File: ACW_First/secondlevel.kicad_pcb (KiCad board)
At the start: 2 copper layers, 103 x 65 mm, 69 parts, among them J11 24VDC, J12 Conn_01x02_Pin, J13 Conn_01x04_Socket, J14 Conn_01x02_Pin, J2 Conn_01x03_Pin, J3 3.8VDC, J4 5VDC, J5 12VDC, U2 MP1584EN, U3 MP1584EN

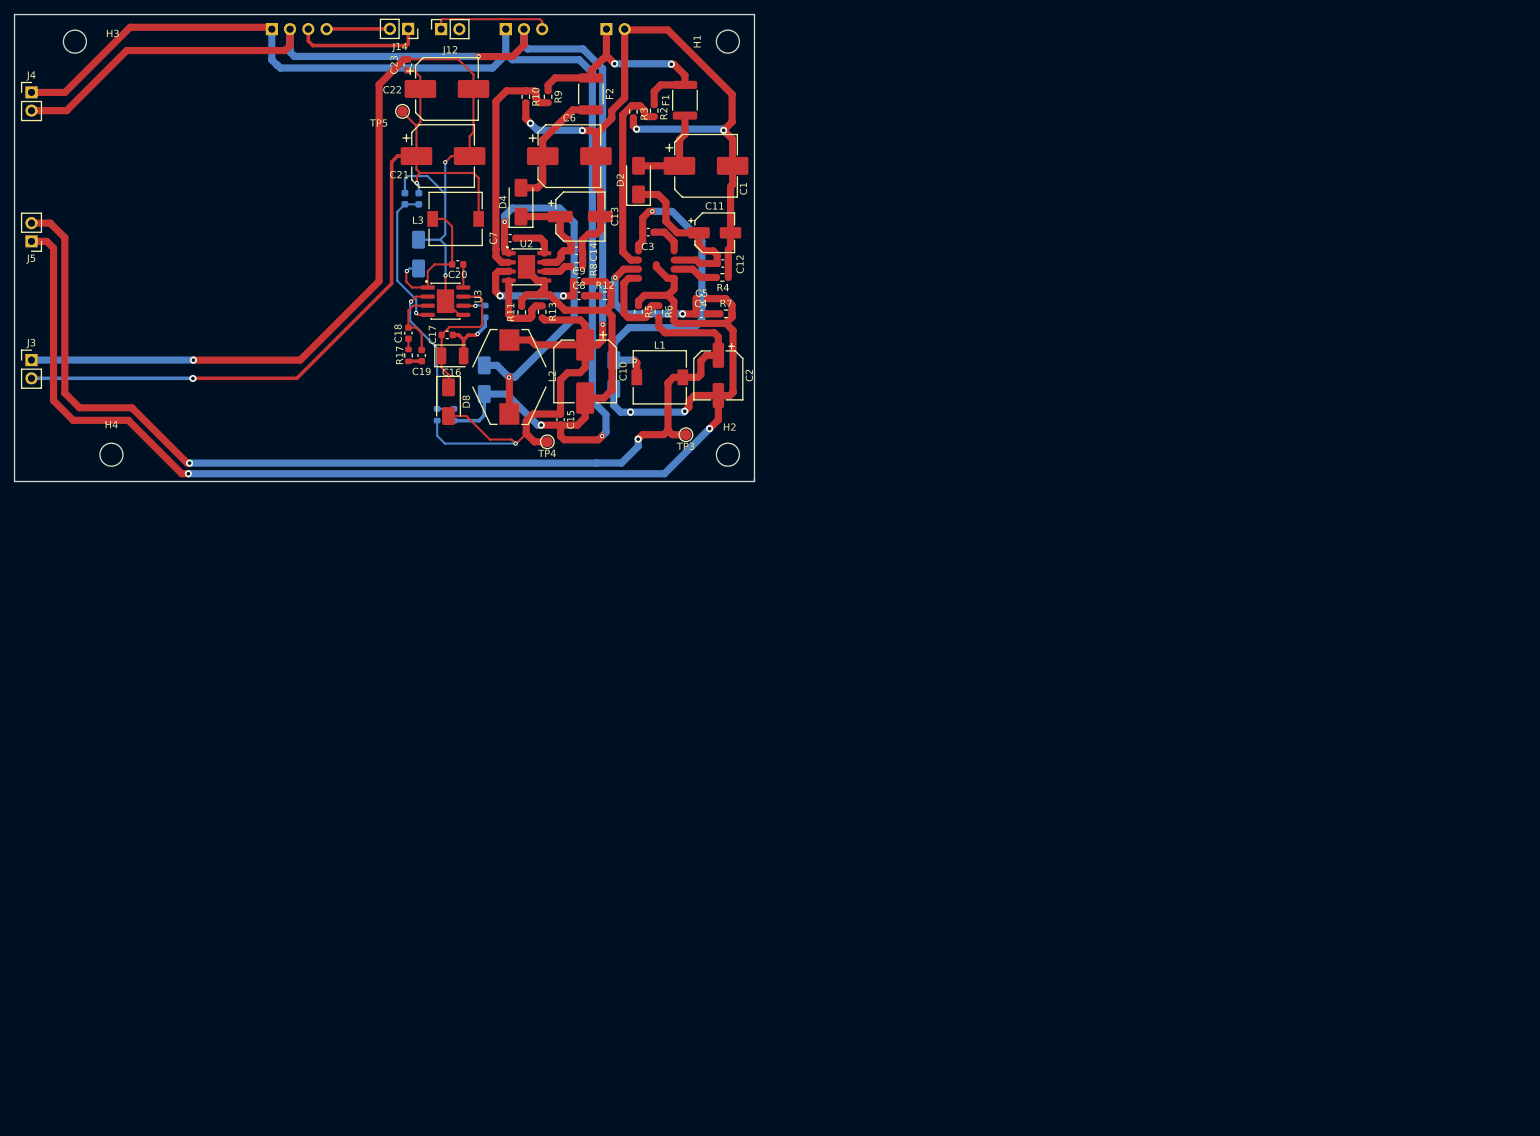
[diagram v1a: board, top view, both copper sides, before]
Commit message: okok
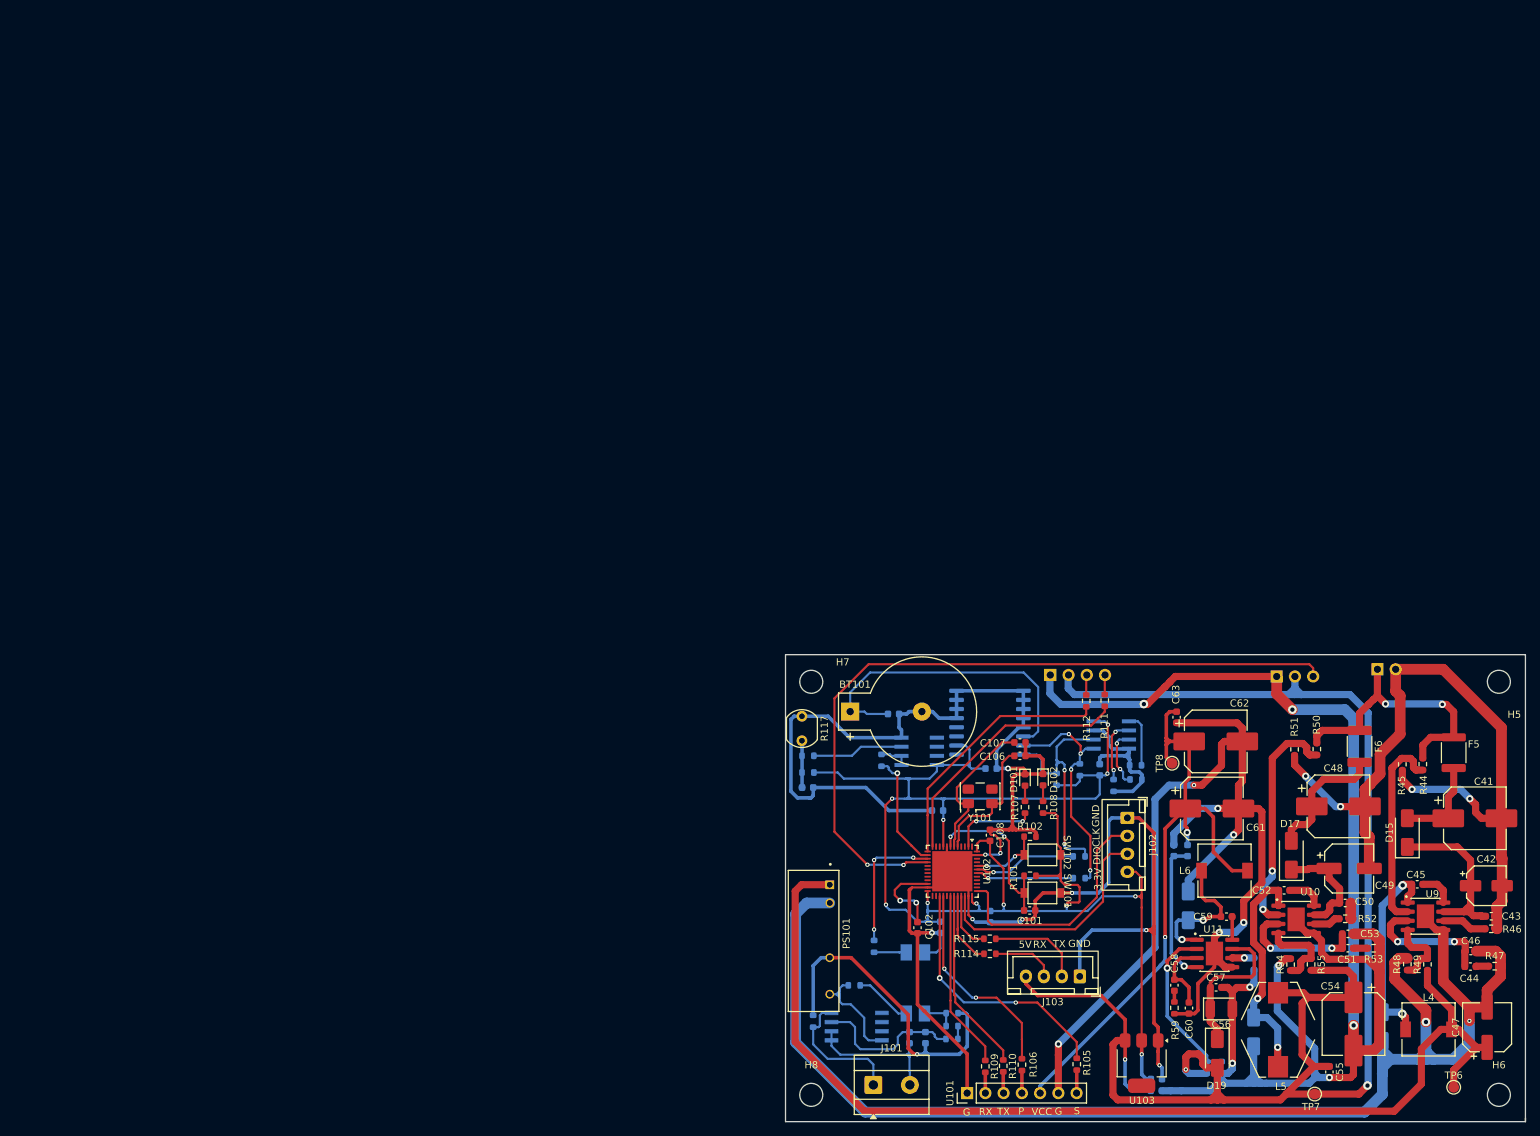
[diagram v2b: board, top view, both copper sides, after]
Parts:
- removed C1, C6: 220µF, Capacitor_SMD:CP_Elec_8x10.5
- removed C10: 470µF, Capacitor_SMD:CP_Elec_8x10.5
- removed C11: 10µF, Capacitor_SMD:CP_Elec_5x5.4
- removed C12, C14, C15, C17, C20, C23, C3, C7: 100nF, Capacitor_SMD:C_0603_1608Metric
- removed C13: 10µF, Capacitor_SMD:CP_Elec_6.3x5.4
- removed C16: 10µF, Capacitor_Tantalum_SMD:CP_EIA-3528-21_Kemet-B
- removed C18, C4, C8: 220pF, Capacitor_SMD:C_0603_1608Metric
- removed C19, C5, C9: NS, Capacitor_SMD:C_0603_1608Metric
- removed C2: 22µF, Capacitor_SMD:CP_Elec_6.3x5.4
- removed C21, C22: 330µF, Capacitor_SMD:CP_Elec_8x10.5
- removed D2, D3, D4, D5, D7, D8: SS34, Diode_SMD:D_SMA
- removed F1: Resettable Fuse/2A, Fuse:Fuse_1812_4532Metric
- removed F2: Resettable Fuse/2A, Fuse:Fuse_1812_4532Metric_Pad1.30x3.40mm_HandSolder
- removed H1, H2, H3, H4: MountingHole, MountingHole:MountingHole_3.2mm_M3
- removed J12, J14: Conn_01x02_Pin, Connector_PinSocket_2.54mm:PinSocket_1x02_P2.54mm_Vertical
- removed J3: 3.8VDC, Connector_PinHeader_2.54mm:PinHeader_1x02_P2.54mm_Vertical
- removed J4: 5VDC, Connector_PinHeader_2.54mm:PinHeader_1x02_P2.54mm_Vertical
- removed J5: 12VDC, Connector_PinHeader_2.54mm:PinHeader_1x02_P2.54mm_Vertical
- removed L1: 22µH, Inductor_SMD:L_7.3x7.3_H4.5
- removed L2: 10µH, Inductor_SMD:L_Bourns-SRR1005
- removed L3: 10µH, Inductor_SMD:L_7.3x7.3_H4.5
- removed R10: 11KΩ, Resistor_SMD:R_0603_1608Metric
- removed R11, R5: 40.2KΩ, Resistor_SMD:R_0603_1608Metric
- removed R12, R17: 68.1KΩ, Resistor_SMD:R_0603_1608Metric
- removed R13: 210KΩ, Resistor_SMD:R_0603_1608Metric
- removed R14: 20KΩ, Resistor_SMD:R_0603_1608Metric
- removed R15: 10KΩ, Resistor_SMD:R_0603_1608Metric
- removed R16, R4, R8: 200KΩ, Resistor_SMD:R_0603_1608Metric
- removed R18: 150KΩ, Capacitor_SMD:C_0603_1608Metric
- removed R19: 40.2KΩ, Capacitor_SMD:C_0603_1608Metric
- removed R2: 149KΩ/1%, Resistor_SMD:R_0603_1608Metric
- removed R3: 11KΩ/1%, Resistor_SMD:R_0603_1608Metric
- removed R6: 562KΩ, Resistor_SMD:R_0603_1608Metric
- removed R7: 68.1KΩ/1%, Resistor_SMD:R_0603_1608Metric
- removed R9: 149KΩ, Resistor_SMD:R_0603_1608Metric
- removed TP3: 12VTP, TestPoint:TestPoint_Pad_D1.5mm
- removed TP4: 5VTP, TestPoint:TestPoint_Pad_D1.5mm
- removed TP5: 3.8VTP, TestPoint:TestPoint_Pad_D1.5mm
- removed U2, U3: MP1584EN, Custom_Footprints:SOIC127P600X170-9N
- added BT101: Battery_Cell, Battery:BatteryHolder_Keystone_500, F.Cu at (550.6, 238.5)
- added C101: 100nf, Capacitor_SMD:C_0603_1608Metric, F.Cu at (575.6, 266.2)
- added C102: 2.2uf, Capacitor_SMD:C_0603_1608Metric, F.Cu at (559.9, 268.6)
- added C103: 100nf, Capacitor_SMD:C_0603_1608Metric, B.Cu at (593.2, 291.3)
- added C104: 100nf, Capacitor_SMD:C_0603_1608Metric, B.Cu at (563.1, 268.6)
- added C105: 100nf, Capacitor_SMD:C_0603_1608Metric, B.Cu at (570.0, 267.1)
- added C106: 22pf, Capacitor_SMD:C_0603_1608Metric, F.Cu at (574.2, 244.7)
- added C107: 22pf, Capacitor_SMD:C_0603_1608Metric, F.Cu at (574.2, 242.8)
- added C108: 100nf, Capacitor_SMD:C_0603_1608Metric, F.Cu at (570.0, 255.7)
- added C109: 100nf, Capacitor_SMD:C_0603_1608Metric, B.Cu at (593.2, 289.7)
- added C110: 100nf, Capacitor_SMD:C_0603_1608Metric, B.Cu at (562.7, 252.3)
- added C111: 100nf, Capacitor_SMD:C_0603_1608Metric, B.Cu at (544.6, 249.1)
- added C112: 1uf, Capacitor_SMD:C_0603_1608Metric, B.Cu at (570.2, 246.5)
- added C113: 1uf, Capacitor_SMD:C_0603_1608Metric, B.Cu at (585.3, 246.6)
- added C114: 1uf, Capacitor_SMD:C_0603_1608Metric, B.Cu at (556.6, 238.9)
- added C115: 1uf, Capacitor_SMD:C_0603_1608Metric, B.Cu at (561.0, 283.9)
- added C116: 1uf, Capacitor_SMD:C_0603_1608Metric, B.Cu at (558.8, 283.9)
- added C41: 220µF, Capacitor_SMD:CP_Elec_8x10.5, F.Cu at (637.5, 253.4)
- added C42: 10µF, Capacitor_SMD:CP_Elec_5x5.4, F.Cu at (639.1, 262.8)
- added C43: 100nF, Capacitor_SMD:C_0603_1608Metric, F.Cu at (639.8, 267.0)
- added C44: 220pF, Capacitor_SMD:C_0603_1608Metric, F.Cu at (636.9, 274.0)
- added C45: 100nF, Capacitor_SMD:C_0603_1608Metric, F.Cu at (629.5, 262.6)
- added C46: NS, Capacitor_SMD:C_0603_1608Metric, F.Cu at (637.0, 271.9)
- added C47: 22µF, Capacitor_SMD:CP_Elec_6.3x5.4, F.Cu at (639.2, 282.5)
- added C48: 220µF, Capacitor_SMD:CP_Elec_8x10.5, F.Cu at (618.5, 251.7)
- added C49: 10µF, Capacitor_SMD:CP_Elec_6.3x5.4, F.Cu at (620.0, 260.4)
- added C50: 100nF, Capacitor_SMD:C_0603_1608Metric, F.Cu at (619.5, 265.2)
- added C51: 220pF, Capacitor_SMD:C_0603_1608Metric, F.Cu at (619.9, 271.5)
- added C52: 100nF, Capacitor_SMD:C_0603_1608Metric, F.Cu at (611.0, 263.4)
- added C53: NS, Capacitor_SMD:C_0603_1608Metric, F.Cu at (619.9, 269.5)
- added C54: 470µF, Capacitor_SMD:CP_Elec_8x10.5, F.Cu at (620.6, 282.0)
- added C55: 100nF, Capacitor_SMD:C_0603_1608Metric, F.Cu at (617.3, 288.7)
- added C56: 10µF, Capacitor_Tantalum_SMD:CP_EIA-3528-21_Kemet-B, F.Cu at (602.2, 279.9)
- added C57: 100nF, Capacitor_SMD:C_0603_1608Metric, F.Cu at (601.5, 276.9)
- added C58: 220pF, Capacitor_SMD:C_0603_1608Metric, F.Cu at (595.7, 276.6)
- added C59: 100nF, Capacitor_SMD:C_0603_1608Metric, F.Cu at (603.0, 267.1)
- added C60: NS, Capacitor_SMD:C_0603_1608Metric, F.Cu at (597.7, 279.8)
- added C61: 330µF, Capacitor_SMD:CP_Elec_8x10.5, F.Cu at (600.9, 252.0)
- added C62: 330µF, Capacitor_SMD:CP_Elec_8x10.5, F.Cu at (601.5, 242.7)
- added C63: 100nF, Capacitor_SMD:C_0603_1608Metric, F.Cu at (596.0, 239.3)
- added D101: LED, LED_SMD:LED_0603_1608Metric, F.Cu at (574.9, 248.0)
- added D102: LED, LED_SMD:LED_0603_1608Metric, F.Cu at (577.4, 248.0)
- added D15: SS34, Diode_SMD:D_SMA, F.Cu at (628.1, 255.4)
- added D16: SS34, Diode_SMD:D_SMA, B.Cu at (624.6, 282.4)
- added D17: SS34, Diode_SMD:D_SMA, F.Cu at (612.0, 258.5)
- added D18: SS34, Diode_SMD:D_SMA, B.Cu at (606.7, 283.1)
- added D19: SS34, Diode_SMD:D_SMA, F.Cu at (601.7, 286.1)
- added D20: SS34, Diode_SMD:D_SMA, B.Cu at (597.6, 265.6)
- added F5: Resettable Fuse/2A, Fuse:Fuse_1812_4532Metric, F.Cu at (634.6, 244.2)
- added F6: Resettable Fuse/2A, Fuse:Fuse_1812_4532Metric_Pad1.30x3.40mm_HandSolder, F.Cu at (621.5, 243.4)
- added H5: MountingHole, MountingHole:MountingHole_3.2mm_M3, F.Cu at (640.9, 234.4)
- added H6: MountingHole, MountingHole:MountingHole_3.2mm_M3, F.Cu at (640.9, 291.9)
- added H7: MountingHole, MountingHole:MountingHole_3.2mm_M3, F.Cu at (545.2, 234.4)
- added H8: MountingHole, MountingHole:MountingHole_3.2mm_M3, F.Cu at (545.2, 291.9)
- added J101: Conn_01x02_Male, TerminalBlock_MetzConnect:TerminalBlock_MetzConnect_Type101_RT01602HBWC_1x02_P5.08mm_Horizontal, F.Cu at (553.8, 290.5)
- added J102: Conn_STLink, Connector_JST:JST_XH_B4B-XH-A_1x04_P2.50mm_Vertical, F.Cu at (589.1, 253.3)
- added J103: Conn_01x04_Female, Connector_JST:JST_XH_B4B-XH-A_1x04_P2.50mm_Vertical, F.Cu at (582.5, 275.4)
- added L4: 22µH, Inductor_SMD:L_7.3x7.3_H4.5, F.Cu at (631.1, 282.8)
- added L5: 10µH, Inductor_SMD:L_Bourns-SRR1005, F.Cu at (610.1, 282.8)
- added L6: 10µH, Inductor_SMD:L_7.3x7.3_H4.5, F.Cu at (602.7, 260.7)
- added PS101: RKZ-1212S_P, Custom_Library:CONV_RKZ-1212S_P, F.Cu at (545.5, 270.5)
- added R101: 10k, Resistor_SMD:R_0603_1608Metric, F.Cu at (575.6, 261.4)
- added R102: 10k, Resistor_SMD:R_0603_1608Metric, F.Cu at (575.6, 255.9)
- added R103: 100, Resistor_SMD:R_0603_1608Metric, B.Cu at (582.5, 261.7)
- added R104: 100, Resistor_SMD:R_0603_1608Metric, B.Cu at (582.4, 258.7)
- added R105: 100, Resistor_SMD:R_0603_1608Metric, F.Cu at (582.1, 287.6)
- added R106: 100, Resistor_SMD:R_0603_1608Metric, F.Cu at (574.5, 287.7)
- added R107: 220, Resistor_SMD:R_0603_1608Metric, F.Cu at (574.9, 251.8)
- added R108: 220, Resistor_SMD:R_0603_1608Metric, F.Cu at (577.4, 251.8)
- added R109: 100, Resistor_SMD:R_0603_1608Metric, F.Cu at (569.4, 287.9)
- added R110: 100, Resistor_SMD:R_0603_1608Metric, F.Cu at (571.9, 287.8)
- added R111: 100, Resistor_SMD:R_0603_1608Metric, F.Cu at (586.0, 237.0)
- added R112: 100, Resistor_SMD:R_0603_1608Metric, F.Cu at (583.4, 237.0)
- added R113: 100, Resistor_SMD:R_0603_1608Metric, B.Cu at (554.9, 245.3)
- added R114: 100, Resistor_SMD:R_0603_1608Metric, F.Cu at (570.0, 272.2)
- added R115: 100, Resistor_SMD:R_0603_1608Metric, F.Cu at (570.0, 270.2)
- added R116: 10k, Resistor_SMD:R_0603_1608Metric, B.Cu at (544.7, 247.0)
- added R117: LDR07, OptoDevice:R_LDR_5.1x4.3mm_P3.4mm_Vertical, F.Cu at (543.9, 242.6)
- added R118: 220, Resistor_SMD:R_0603_1608Metric, B.Cu at (544.7, 244.7)
- added R119: 4.7k, Resistor_SMD:R_0603_1608Metric, B.Cu at (590.4, 248.0)
- added R120: 4.7k, Resistor_SMD:R_0603_1608Metric, B.Cu at (587.2, 248.8)
- added R121: 4.7k, Resistor_SMD:R_0603_1608Metric, B.Cu at (590.3, 246.0)
- added R122: 4.7k, Resistor_SMD:R_0603_1608Metric, B.Cu at (582.5, 246.6)
- added R123: 4.7k, Resistor_SMD:R_0603_1608Metric, B.Cu at (579.3, 248.0)
- added R124: 220, Resistor_SMD:R_0603_1608Metric, B.Cu at (553.9, 271.2)
- added R125: 10k, Resistor_SMD:R_0603_1608Metric, B.Cu at (551.1, 276.6)
- added R126: 4.7k, Resistor_SMD:R_0603_1608Metric, B.Cu at (564.8, 280.5)
- added R127: 10k, Resistor_SMD:R_0603_1608Metric, B.Cu at (564.8, 282.3)
- added R128: 10k, Resistor_SMD:R_0603_1608Metric, B.Cu at (564.7, 284.1)
- added R129: 4.7k, Resistor_SMD:R_0603_1608Metric, B.Cu at (545.4, 281.6)
- added R44: 149KΩ/1%, Resistor_SMD:R_0603_1608Metric, F.Cu at (630.3, 245.8)
- added R45: 11KΩ/1%, Resistor_SMD:R_0603_1608Metric, F.Cu at (627.4, 245.9)
- added R46: 200KΩ, Resistor_SMD:R_0603_1608Metric, F.Cu at (639.8, 268.8)
- added R47: 68.1KΩ/1%, Resistor_SMD:R_0603_1608Metric, F.Cu at (640.3, 274.0)
- added R48: 40.2KΩ, Resistor_SMD:R_0603_1608Metric, F.Cu at (628.1, 273.7)
- added R49: 562KΩ, Resistor_SMD:R_0603_1608Metric, F.Cu at (630.9, 273.7)
- added R50: 149KΩ, Resistor_SMD:R_0603_1608Metric, F.Cu at (615.5, 243.7)
- added R51: 11KΩ, Resistor_SMD:R_0603_1608Metric, F.Cu at (612.4, 243.8)
- added R52: 200KΩ, Resistor_SMD:R_0603_1608Metric, F.Cu at (619.5, 267.4)
- added R53: 68.1KΩ, Resistor_SMD:R_0603_1608Metric, F.Cu at (623.4, 271.5)
- added R54: 40.2KΩ, Resistor_SMD:R_0603_1608Metric, F.Cu at (611.9, 273.7)
- added R55: 210KΩ, Resistor_SMD:R_0603_1608Metric, F.Cu at (614.7, 273.7)
- added R56: 20KΩ, Resistor_SMD:R_0603_1608Metric, B.Cu at (600.2, 288.1)
- added R57: 10KΩ, Resistor_SMD:R_0603_1608Metric, B.Cu at (602.3, 288.1)
- added R58: 200KΩ, Resistor_SMD:R_0603_1608Metric, B.Cu at (606.8, 273.6)
- added R59: 68.1KΩ, Resistor_SMD:R_0603_1608Metric, F.Cu at (595.7, 279.8)
- added R60: 40.2KΩ, Capacitor_SMD:C_0603_1608Metric, B.Cu at (595.6, 257.9)
- added R61: 150KΩ, Capacitor_SMD:C_0603_1608Metric, B.Cu at (597.5, 257.9)
- added SW101: SW_Push, Library:Pushbutton_3x4x2mm_2P_SMD, F.Cu at (577.3, 261.3)
- added SW102: SW_Push, Library:Pushbutton_3x4x2mm_2P_SMD, F.Cu at (577.3, 256.0)
- added TP6: 12VTP, TestPoint:TestPoint_Pad_D1.5mm, F.Cu at (634.6, 290.8)
- added TP7: 5VTP, TestPoint:TestPoint_Pad_D1.5mm, F.Cu at (615.2, 291.8)
- added TP8: 3.8VTP, TestPoint:TestPoint_Pad_D1.5mm, F.Cu at (595.4, 245.7)
- added U10: MP1584EN, Custom_Footprints:SOIC127P600X170-9N, F.Cu at (612.7, 267.5)
- added U101: A7600_Pinout, Connector_PinHeader_2.54mm:PinHeader_1x07_P2.54mm_Vertical, F.Cu at (566.9, 291.6)
- added U102: STM32F401CCUx, Package_DFN_QFN:QFN-48-1EP_7x7mm_P0.5mm_EP5.6x5.6mm, F.Cu at (564.8, 260.8)
- added U103: AMS1117-3.3, Package_TO_SOT_SMD:SOT-223, F.Cu at (591.1, 287.5)
- added U104: MCP6002-I_SN, Custom_Library:SOIC127P600X175-8N, B.Cu at (560.2, 244.1)
- added U105: DS3231M, Package_SO:SOIC-16W_7.5x10.3mm_P1.27mm, B.Cu at (570.0, 240.1)
- added U106: AT24C512-SSHM, Custom_Library:SOIC127P600X175-8N, B.Cu at (586.9, 241.8)
- added U107: PC817, Custom_Library:SOP254P975X460-4N, B.Cu at (559.6, 276.3)
- added U108: LM358PSR, Custom_Library:SOIC127P780X200-8N, B.Cu at (551.5, 282.4)
- added U11: MP1584EN, Custom_Footprints:SOIC127P600X170-9N, F.Cu at (601.3, 272.2)
- added U9: MP1584EN, Custom_Footprints:SOIC127P600X170-9N, F.Cu at (630.7, 267.0)
- added Y101: 8Mhz, Crystal:Crystal_SMD_5032-4Pin_5.0x3.2mm, F.Cu at (568.7, 250.3)
- moved J13 140.8 mm to (578.4, 233.4)
- moved J2 140.1 mm to (609.9, 233.6)
- moved J11 139.5 mm to (624.0, 232.6)
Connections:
- net /5VDC renamed 5VDC
- J13 pad 3: Net-(J13-Pin_3) -> /PZEM_TXD
- J13 pad 4: Net-(J13-Pin_4) -> /PZEM_RXD
- J2 pad 3: Net-(J12-Pin_1) -> /RELAY_DATA
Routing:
- net GND: track 674.8 -> 971.0 mm, vias 14 -> 28
- net +3.3V: track 0.00 -> 225.2 mm, vias 0 -> 11
- net 12VDC: track 0.00 -> 151.6 mm
- net /24VDC to 12VDC/12VDC: track 149.4 -> 0.00 mm, vias 2 -> 0
- net /5VDC to 3.8VDC/3.8VDC: track 112.4 -> 0.00 mm, vias 2 -> 0
- net /RELAY_DATA: track 0.00 -> 103.7 mm, vias 0 -> 2
- net 3.8VDC: track 0.00 -> 91.1 mm, vias 0 -> 2
- net Net-(D5-K): track 51.4 -> 0.00 mm, vias 2 -> 0
- net Net-(D3-K): track 47.5 -> 0.00 mm, vias 2 -> 0
- net IGND: track 0.00 -> 45.6 mm, vias 0 -> 1
- net Net-(BT101-+): track 0.00 -> 44.7 mm
- net Net-(U102-PB14): track 0.00 -> 36.5 mm, vias 0 -> 2
- net Net-(U102-PA2): track 0.00 -> 36.4 mm
- net Net-(U102-PA3): track 0.00 -> 36.2 mm
- net /Controller/SWDIO: track 0.00 -> 34.2 mm
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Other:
- board text added: "3.3V"
- board text added: "5V"
- board text added: "CLK"
- board text added: "DIO"
- board text added: "G"
- board text added: "GND"
- board text added: "P"
- board text added: "RX"
- board text added: "S"
- board text added: "TX"
- board text added: "VCC"
